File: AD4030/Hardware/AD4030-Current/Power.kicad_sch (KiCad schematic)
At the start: 49 parts, among them J501 1715721, Q501 SI5618A, Q502 MMBT3904, U501 ADP7142AUJZ-1.8, U502 TSR_1-2433, U503 TEC3-2419WI, U504 LT1763CDE-ADJ, U505 LM1117LD-3.3, U506 ADP5070AREZ, U507 ADP7182AUJZ, U508 ADP7142AUJZ, U509 LM1117LD-ADJ, U510 ADP7142AUJZ-1.8

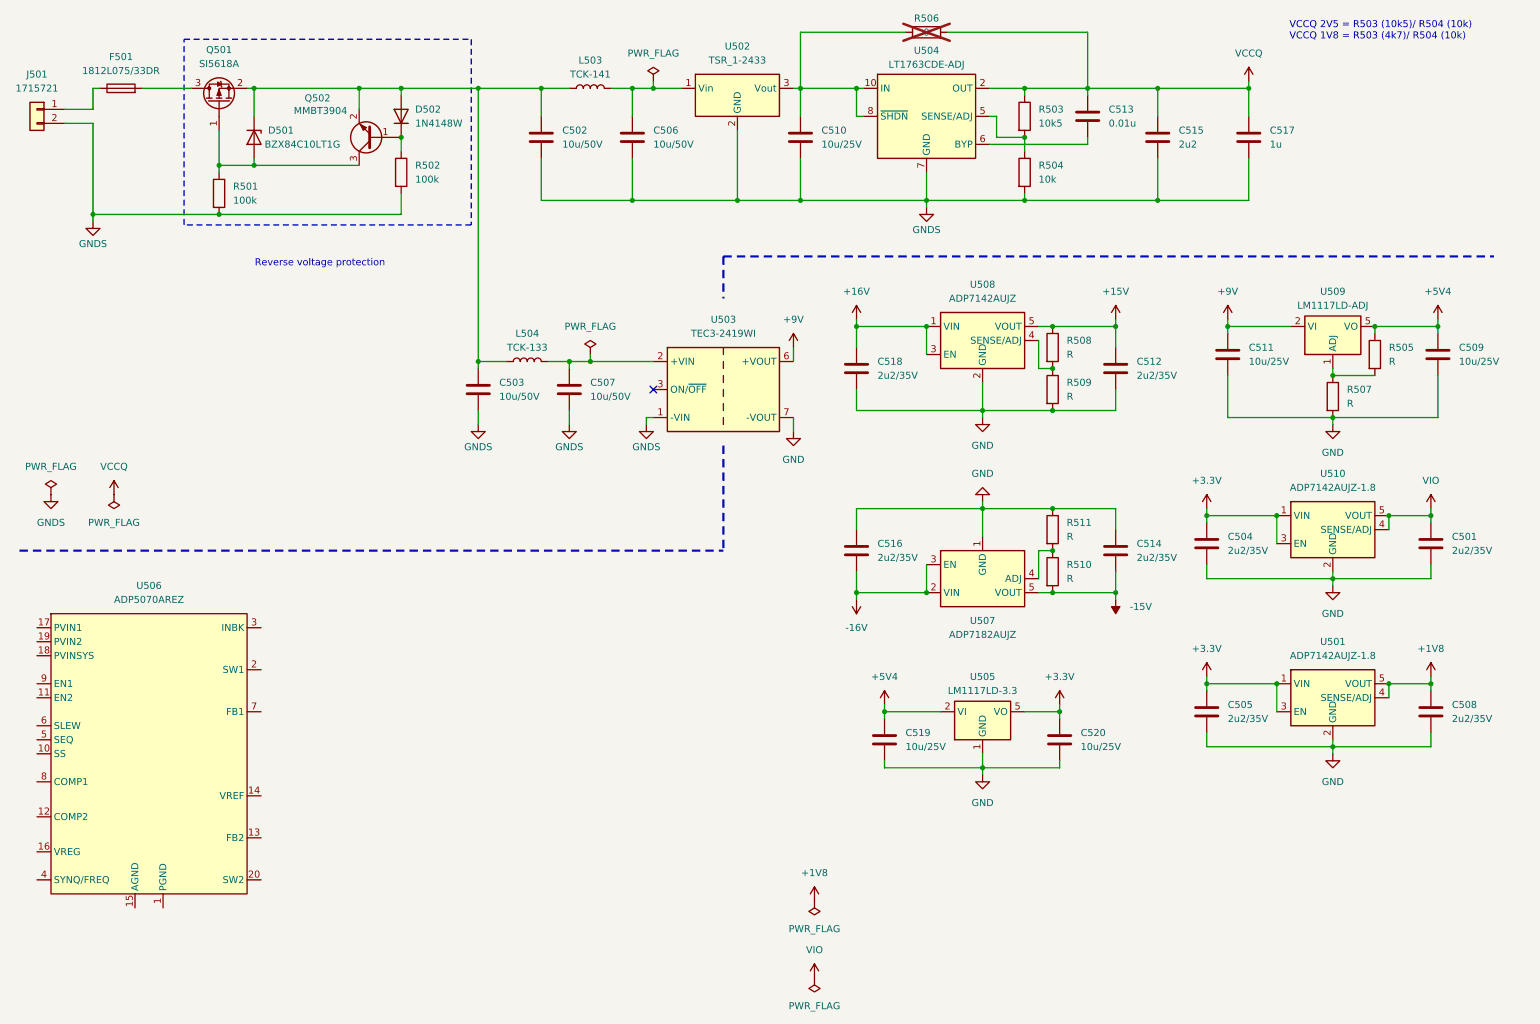
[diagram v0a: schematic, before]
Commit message: Hardware
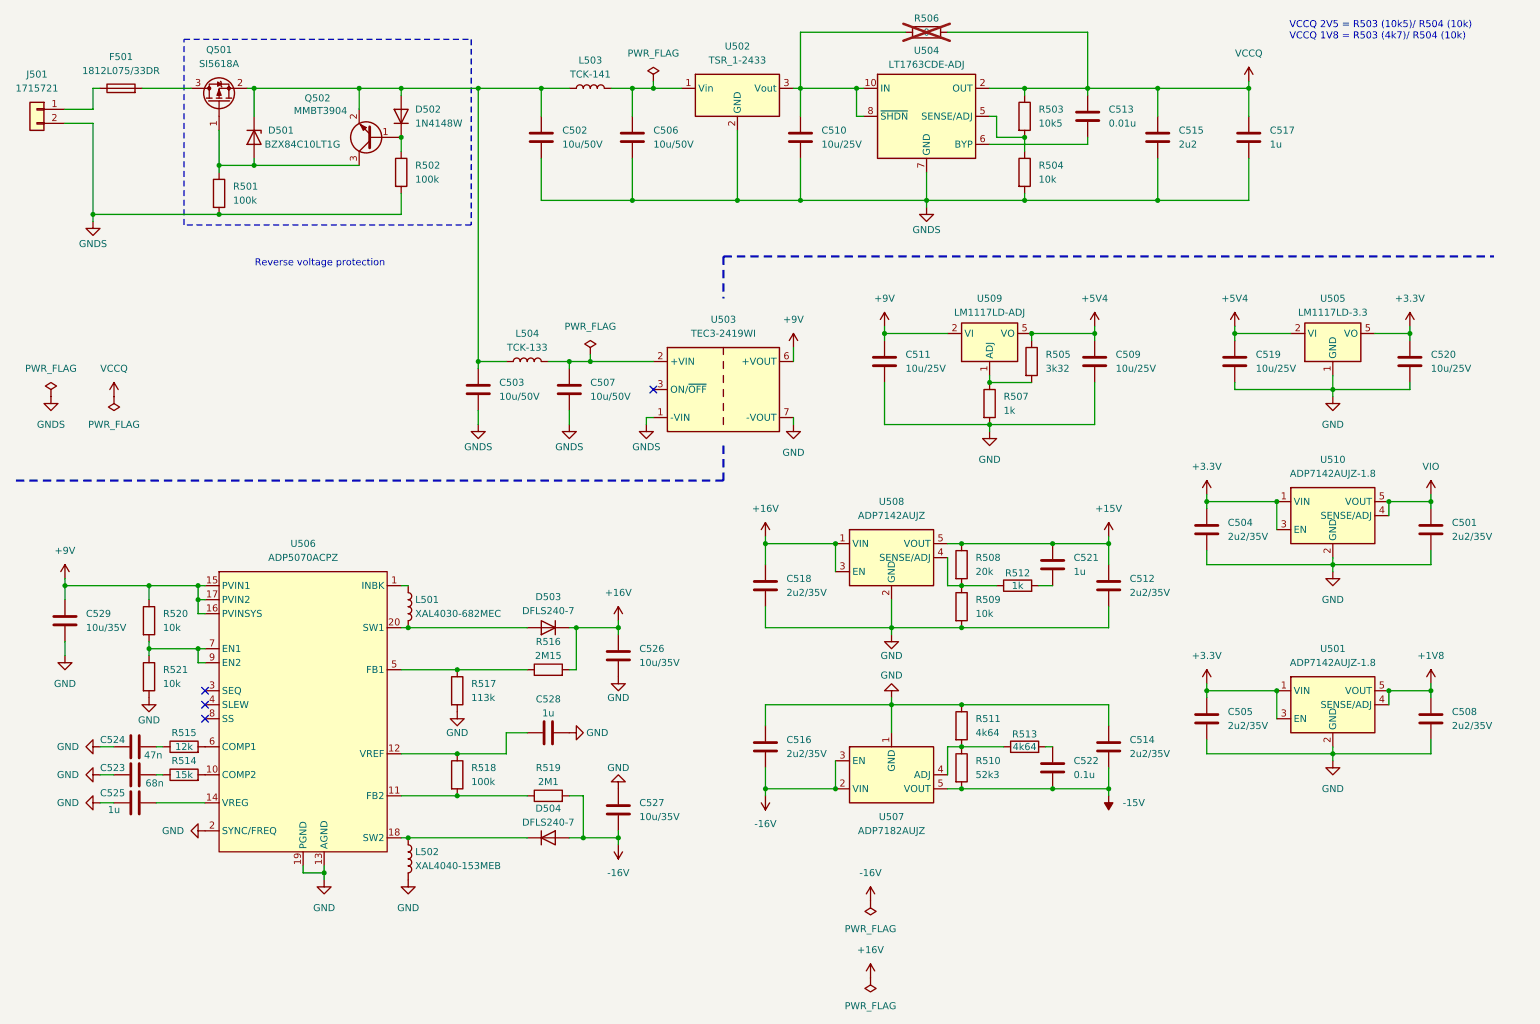
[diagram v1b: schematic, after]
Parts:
- removed U506: ADP5070AREZ, Package_SO:ETSSOP-20-1EP_4.4x6.5mm_P0.65mm_EP3x4.2mm, symbol AD4030:ADP5070AREZ
- added C521, C525, C528: 1u, Capacitor_SMD:C_0603_1608Metric_Pad1.08x0.95mm_HandSolder, symbol Device:C
- added C522: 0.1u, Capacitor_SMD:C_0603_1608Metric_Pad1.08x0.95mm_HandSolder, symbol Device:C
- added C523: 68n, Capacitor_SMD:C_0603_1608Metric_Pad1.08x0.95mm_HandSolder, symbol Device:C
- added C524: 47n, Capacitor_SMD:C_0603_1608Metric_Pad1.08x0.95mm_HandSolder, symbol Device:C
- added C526, C527, C529: 10u/35V, Capacitor_SMD:C_1206_3216Metric_Pad1.33x1.80mm_HandSolder, symbol Device:C
- added D503, D504: DFLS240-7, AD4030:POWERDI123_DIO, symbol Device:D
- added L501: XAL4030-682MEC, Inductor_SMD:L_Coilcraft_XAL4030-XXX, symbol Device:L
- added L502: XAL4040-153MEB, Inductor_SMD:L_Coilcraft_XAL4040-XXX, symbol Device:L
- added R512: 1k, Resistor_SMD:R_0603_1608Metric_Pad0.98x0.95mm_HandSolder, symbol Device:R
- added R513: 4k64, Resistor_SMD:R_0603_1608Metric_Pad0.98x0.95mm_HandSolder, symbol Device:R
- added R514: 15k, Resistor_SMD:R_0603_1608Metric_Pad0.98x0.95mm_HandSolder, symbol Device:R
- added R515: 12k, Resistor_SMD:R_0603_1608Metric_Pad0.98x0.95mm_HandSolder, symbol Device:R
- added R516: 2M15, Resistor_SMD:R_0603_1608Metric_Pad0.98x0.95mm_HandSolder, symbol Device:R
- added R517: 113k, Resistor_SMD:R_0603_1608Metric_Pad0.98x0.95mm_HandSolder, symbol Device:R
- added R518: 100k, Resistor_SMD:R_0603_1608Metric_Pad0.98x0.95mm_HandSolder, symbol Device:R
- added R519: 2M1, Resistor_SMD:R_0603_1608Metric_Pad0.98x0.95mm_HandSolder, symbol Device:R
- added R520, R521: 10k, Resistor_SMD:R_0603_1608Metric_Pad0.98x0.95mm_HandSolder, symbol Device:R
- added U506: ADP5070ACPZ, Package_DFN_QFN:QFN-20-1EP_4x4mm_P0.5mm_EP2.6x2.6mm_ThermalVias, symbol AD4030:ADP5070ACPZ
- R505: value R -> 3k32
- R507: value R -> 1k
- R508: value R -> 20k
- R509: value R -> 10k
- R510: value R -> 52k3
- R511: value R -> 4k64
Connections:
- net +15V: now also C521.1
- net +16V: now also C526.1, D503.1 (K), R516.2
- net +9V: now also C529.1, R520.1, U506.15 (PVIN1), U506.16 (PVINSYS), U506.17 (PVIN2)
- net -15V: now also C522.2
- net -16V: now also C527.2, D504.2 (A), R519.2
- net GND: now also C523.1, C524.1, C525.1, C526.2, C527.1, C528.2, C529.2, L502.2, R517.2, R521.2, U506.13 (AGND), U506.19 (PGND), U506.2 (SYNC/FREQ), U506.21 (AGND)
- net at R508.2, R509.1, U508.4 (SENSE/ADJ): now also R512.1
- net at R510.1, R511.2, U507.4 (ADJ): now also R513.1
- new net: D503.2 (A), L501.2, U506.20 (SW1)
- new net: C522.1, R513.2
- new net: R516.1, R517.1, U506.5 (FB1)
- new net: C523.2, R514.1
- new net: R514.2, U506.10 (COMP2)
- new net: D504.1 (K), L502.1, U506.18 (SW2)
- new net: C528.1, R518.1, U506.12 (VREF)
- new net: R518.2, R519.1, U506.11 (FB2)
- new net: L501.1, U506.1 (INBK)
- new net: R520.2, R521.1, U506.7 (EN1), U506.9 (EN2)
- new net: C521.2, R512.2
- new net: C525.2, U506.14 (VREG)
- new net: R515.2, U506.6 (COMP1)
- new net: C524.2, R515.1
- no-connect marks 1 -> 4
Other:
- moved on the sheet: C501, C504, C505, C508, C509, C511, C512, C514, C516, C518, C519, C520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
